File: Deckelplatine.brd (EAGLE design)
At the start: 110 x 75 mm, 67 parts, among them IC1 MAX1487EESA+, IC2 74HCT595D, IC3 74HCT595D, IC4 74HCT595D, IC5 74HCT595D, IC6 74HCT595D, J1 52808-2570, Q1 BC846BSMD, Q2 BC846BSMD, U1 LM2676S, X1 236-404, X2 233-502

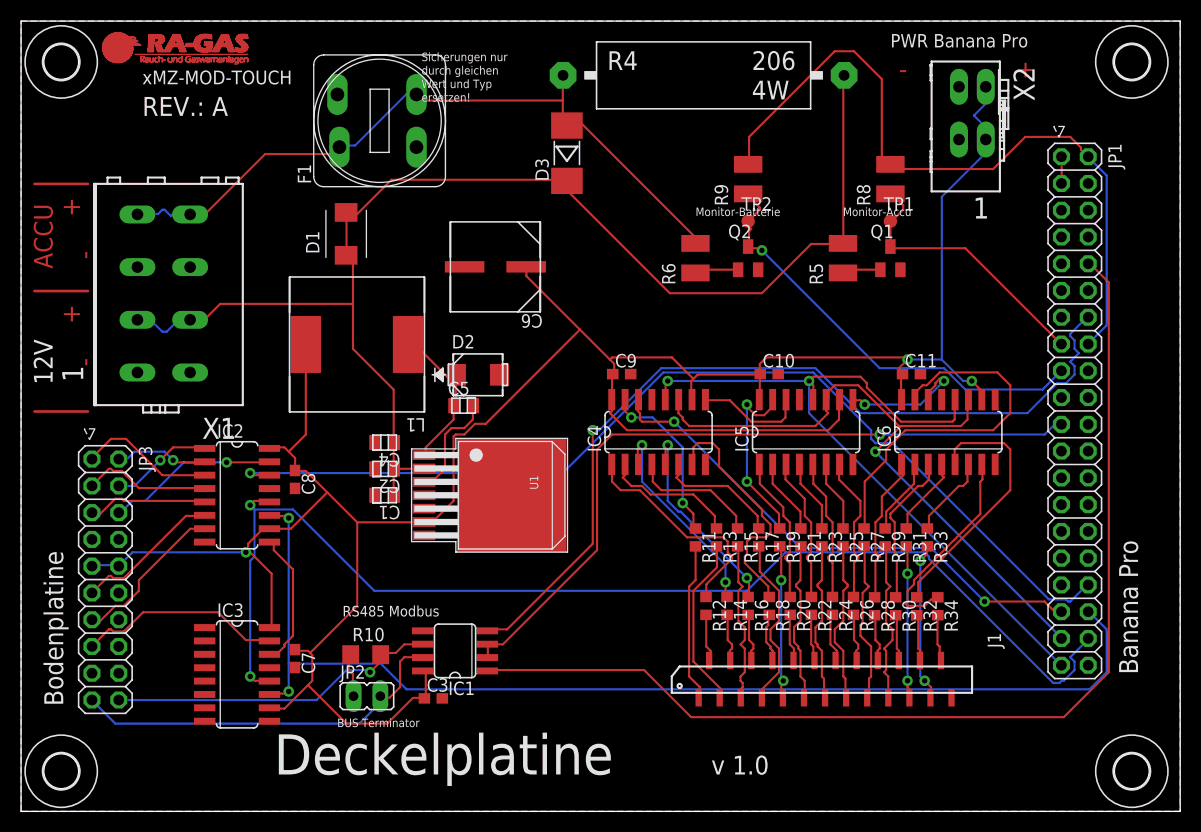
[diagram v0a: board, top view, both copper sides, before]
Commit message: Routing fertig, keine Airwires übrig
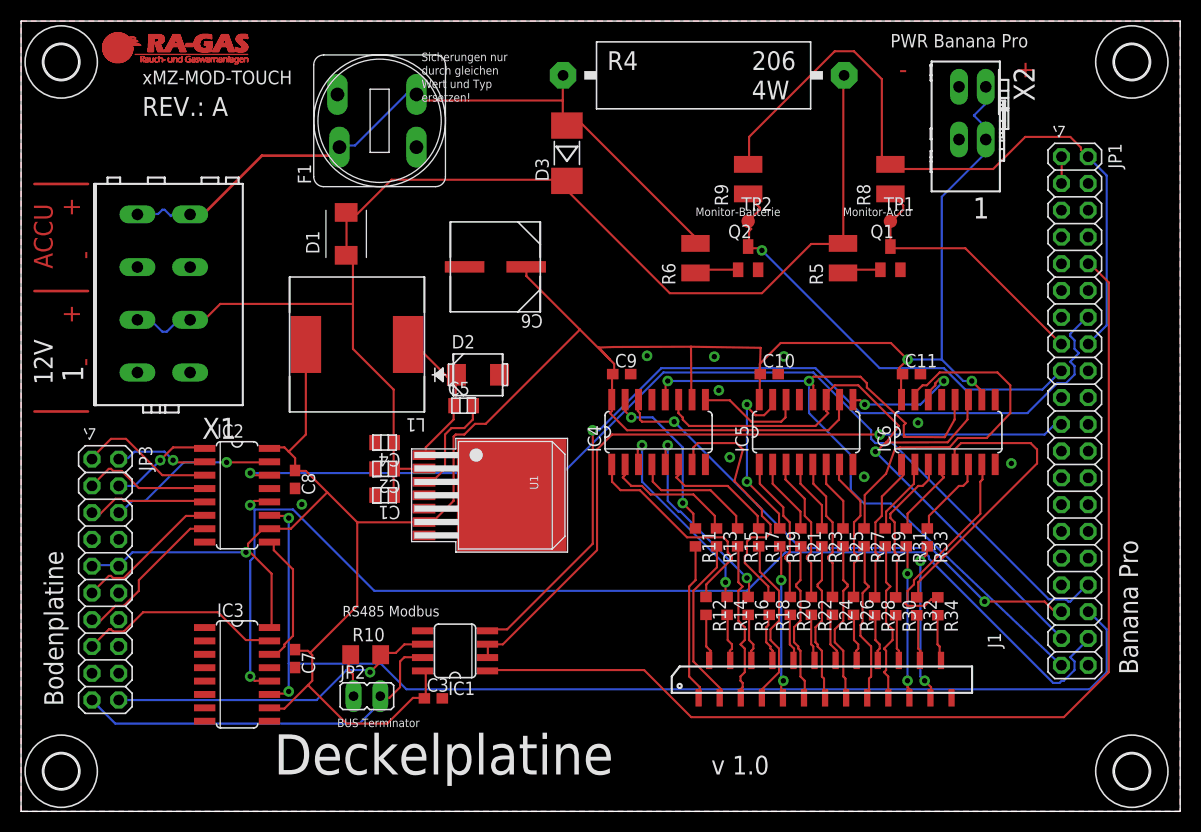
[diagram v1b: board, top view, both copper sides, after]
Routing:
- net VCC: track 249.1 -> 257.3 mm
- net LED_RCK: track 72.1 -> 76.2 mm
- net N$28: track 25.0 -> 28.6 mm
- net LED_SCK: track 64.7 -> 66.5 mm
- net N$13: track 23.3 -> 25.1 mm
- net N$23: track 35.2 -> 34.6 mm
